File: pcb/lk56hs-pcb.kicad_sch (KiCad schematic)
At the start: 9 parts, among them J2 Conn_01x03, J3 Conn_01x05, U1 RaspberryPi_Pico

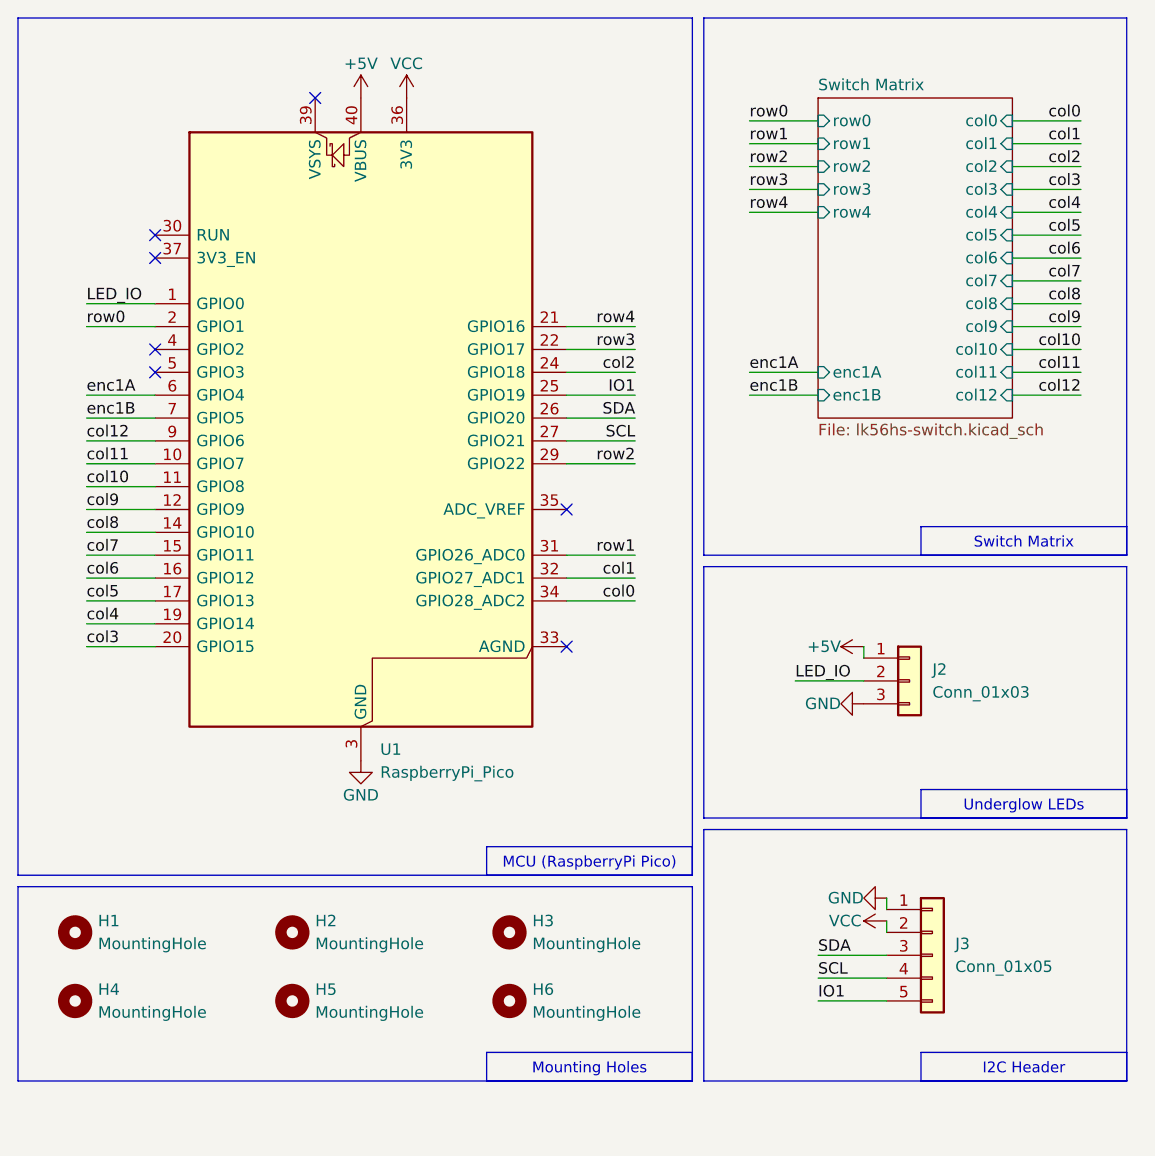
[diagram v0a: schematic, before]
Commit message: Make plate reversible and add graphics
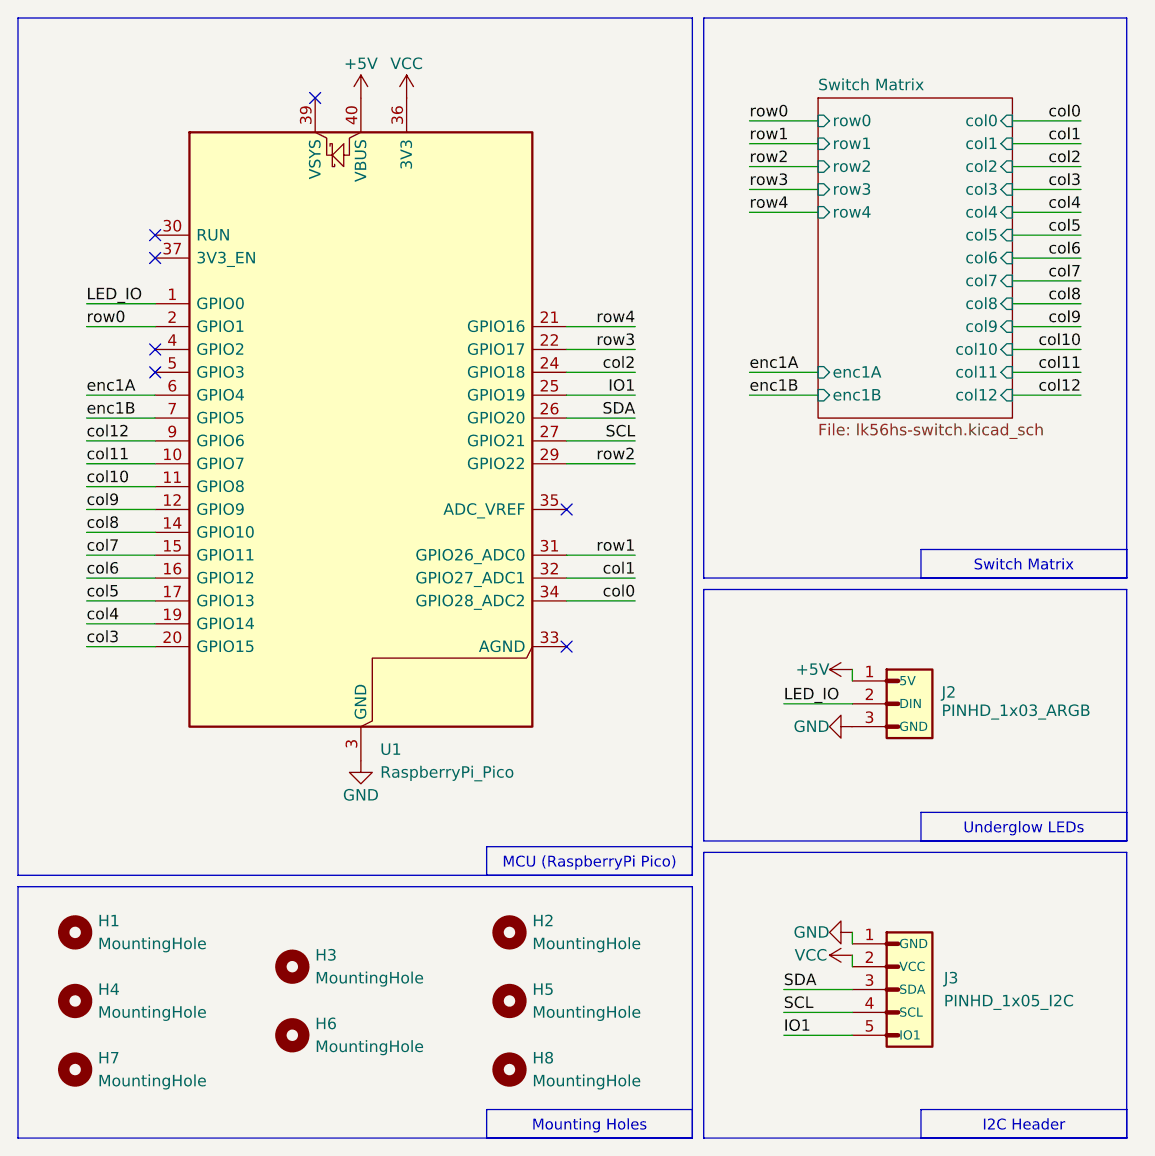
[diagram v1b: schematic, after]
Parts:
- added H7, H8: MountingHole, LKBD_MountingHole:MountingHole_M2_NoPad, symbol Mechanical:MountingHole
- H1: footprint LKBD_MountingHole:MountingHole_M2_NPTH -> LKBD_MountingHole:MountingHole_M2_NoPad
- H2: renamed from H3; footprint LKBD_MountingHole:MountingSlot_M2_Small_NPTH -> LKBD_MountingHole:MountingHole_M2_NoPad
- H3: renamed from H2; footprint LKBD_MountingHole:MountingSlot_M2_NTPH_Half -> LKBD_MountingHole:MountingHole_M2_NoPad
- H4, H6: footprint LKBD_MountingHole:MountingSlot_M2_Small_NPTH -> LKBD_MountingHole:MountingHole_M2_NoPad
- H5: footprint LKBD_MountingHole:MountingSlot_M2_NTPH_Long -> LKBD_MountingHole:MountingHole_M2_NoPad
- J2: value Conn_01x03 -> PINHD_1x03_ARGB; symbol Connector_Generic:Conn_01x03 -> LKBD_Connector:PINHD_1x03_ARGB
- J3: value Conn_01x05 -> PINHD_1x05_I2C; symbol Connector_Generic:Conn_01x05 -> LKBD_Connector:PINHD_1x05_I2C
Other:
- moved on the sheet: H3, H5
